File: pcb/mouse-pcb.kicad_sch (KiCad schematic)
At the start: 7 parts, among them J1 TYPE-C-31-M-12, SW1 D2FC-F-7N20M, SW2 D2FC-F-7N20M, SW3 D2FC-F-7N20M, U1 PAW3395-T6QU, U2 NRF54L15-QFAA-R

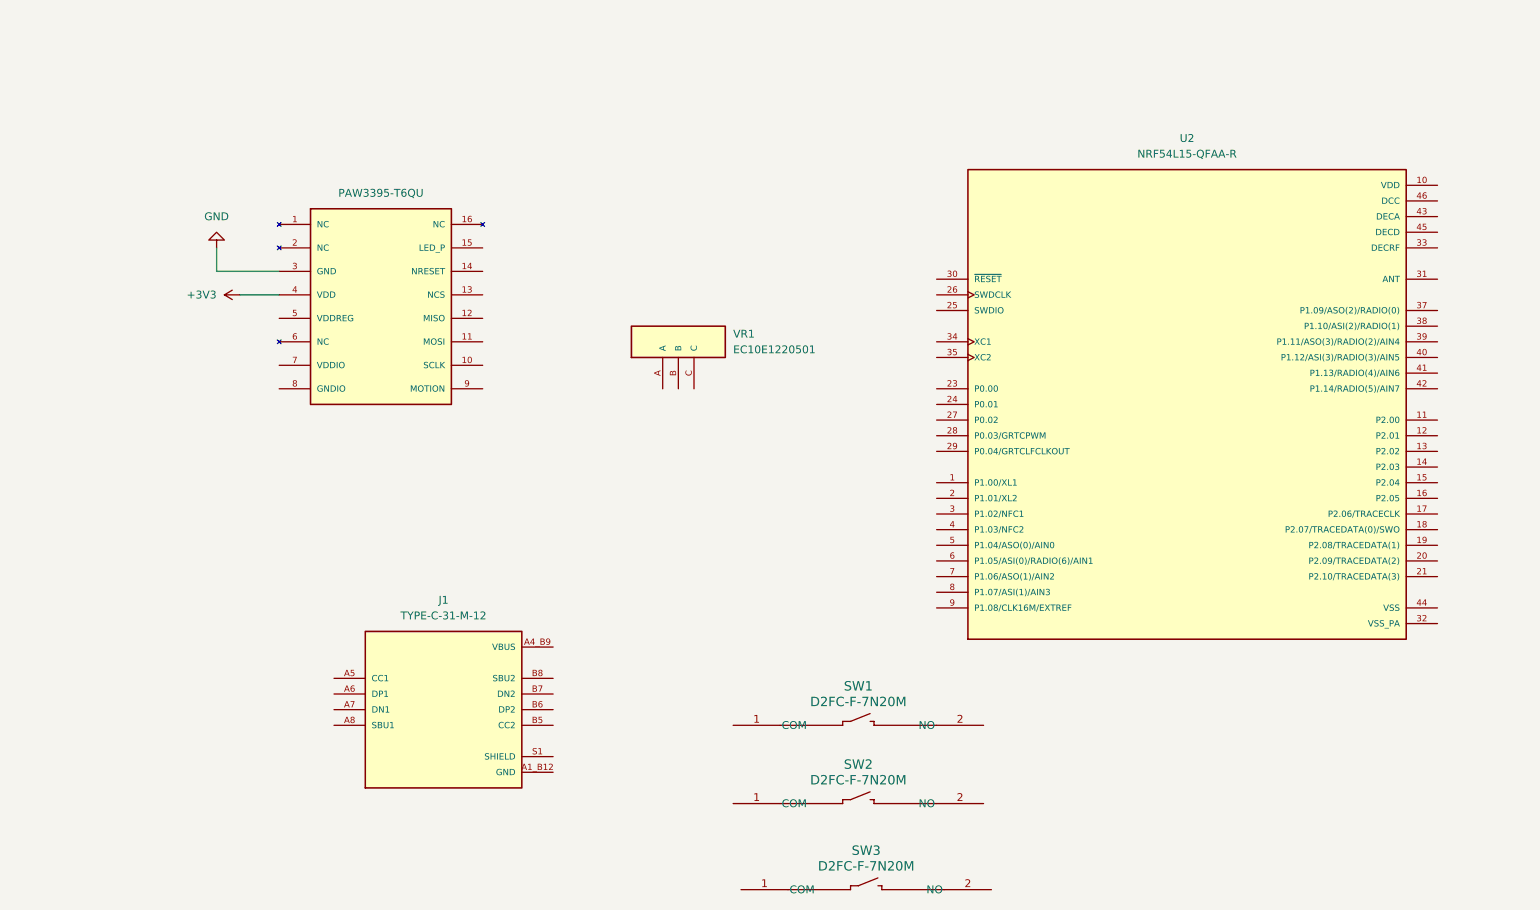
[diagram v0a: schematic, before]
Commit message: feat: adding all the passive for mouse
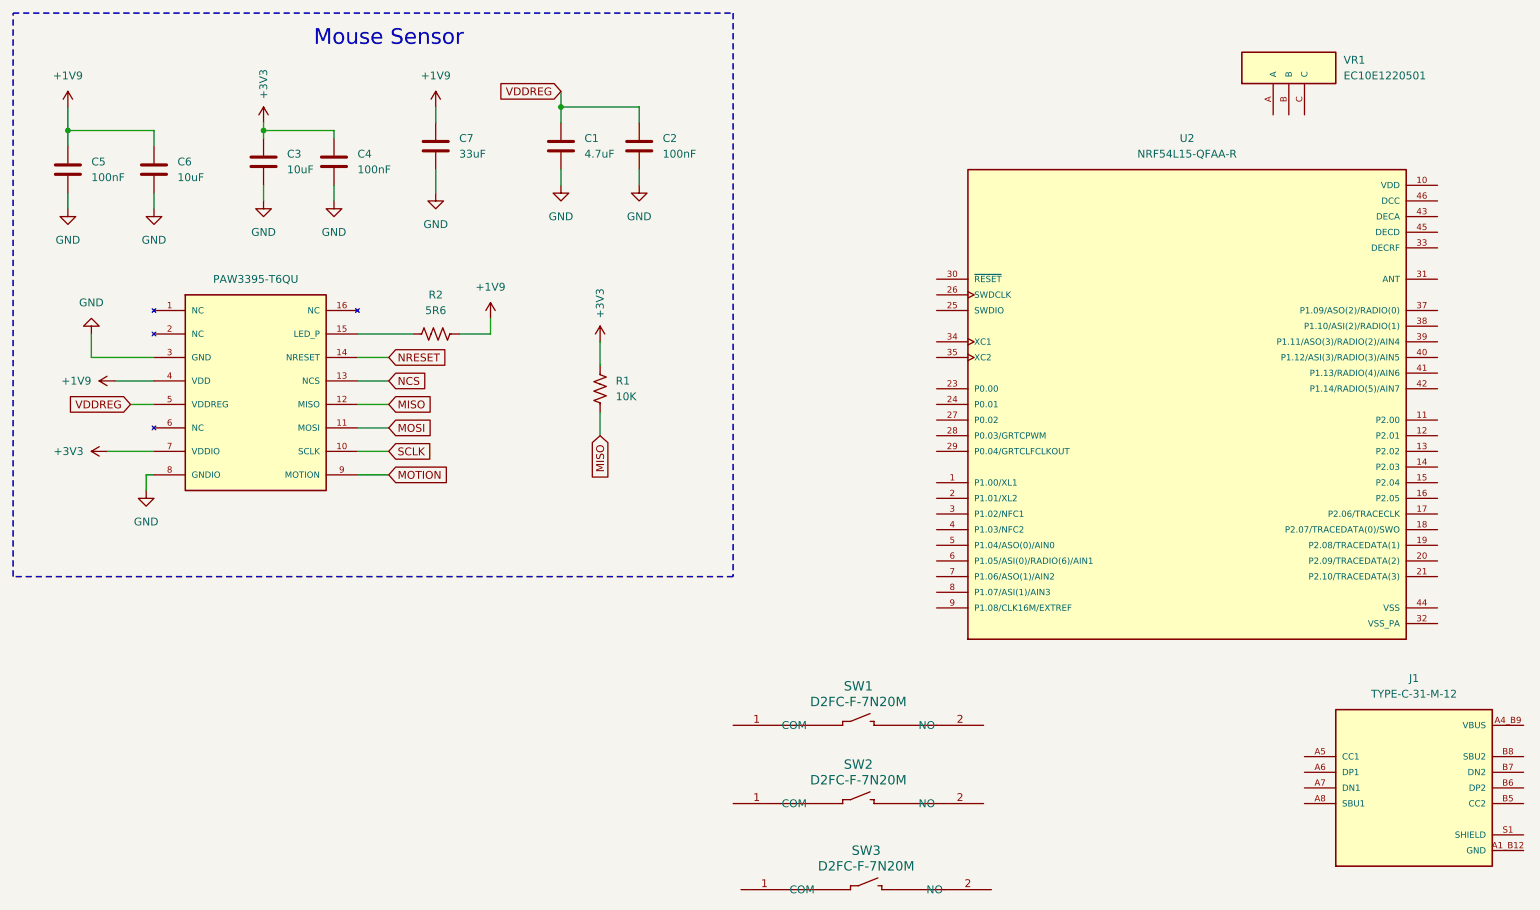
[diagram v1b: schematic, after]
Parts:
- added C1: 4.7uF, Capacitor_SMD:C_0805_2012Metric_Pad1.18x1.45mm_HandSolder, symbol Device:C
- added C2, C4, C5: 100nF, Capacitor_SMD:C_0805_2012Metric_Pad1.18x1.45mm_HandSolder, symbol Device:C
- added C3, C6: 10uF, Capacitor_SMD:C_0805_2012Metric_Pad1.18x1.45mm_HandSolder, symbol Device:C
- added C7: 33uF, Capacitor_SMD:C_0805_2012Metric_Pad1.18x1.45mm_HandSolder, symbol Device:C
- added R1: 10K, Resistor_SMD:R_0805_2012Metric_Pad1.20x1.40mm_HandSolder, symbol Device:R_US
- added R2: 5R6, Resistor_SMD:R_0805_2012Metric_Pad1.20x1.40mm_HandSolder, symbol Device:R_US
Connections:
- net +3V3: now also U1.7 (VDDIO), C3.1, C4.1, R1.1; no longer U1.4 (VDD)
- net GND: now also U1.8 (GNDIO), C1.2, C2.2, C3.2, C4.2, C5.2, C6.2, C7.2
- net SCLK: now reaches U1.10 (SCLK)
- net MOSI: now reaches U1.11 (MOSI)
- net MISO: now reaches U1.12 (MISO)
- net MISO: now also R1.2
- net NCS: now reaches U1.13 (NCS)
- net NRESET: now reaches U1.14 (NRESET)
- net at U1.15 (LED_P): now also R2.1
- net VDDREG: now reaches U1.5 (VDDREG)
- net VDDREG: now also C1.1, C2.1
- net MOTION: now reaches U1.9 (MOTION)
- new net +1V9: C5.1, C6.1, C7.1, R2.2, U1.4 (VDD)
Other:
- note added: "Mouse Sensor"
- moved on the sheet: J1, VR1
